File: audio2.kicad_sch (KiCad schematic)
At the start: 10 parts, among them J10 AudioJack3_SwitchTR, J7 AudioJack3_SwitchTR, U3 LM4950TS

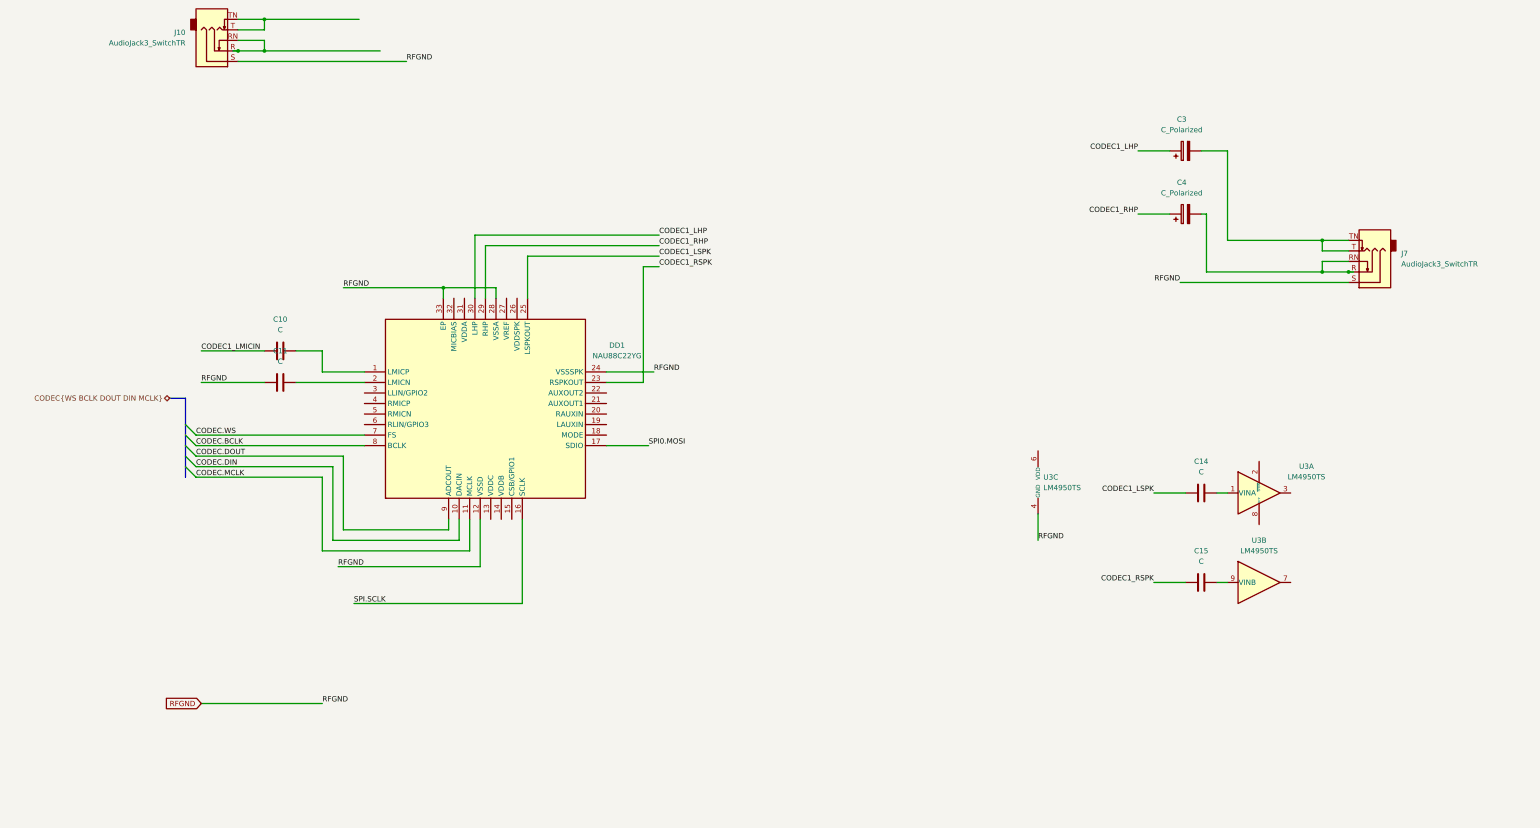
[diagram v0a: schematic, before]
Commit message: Перевёл на иерархические схемы
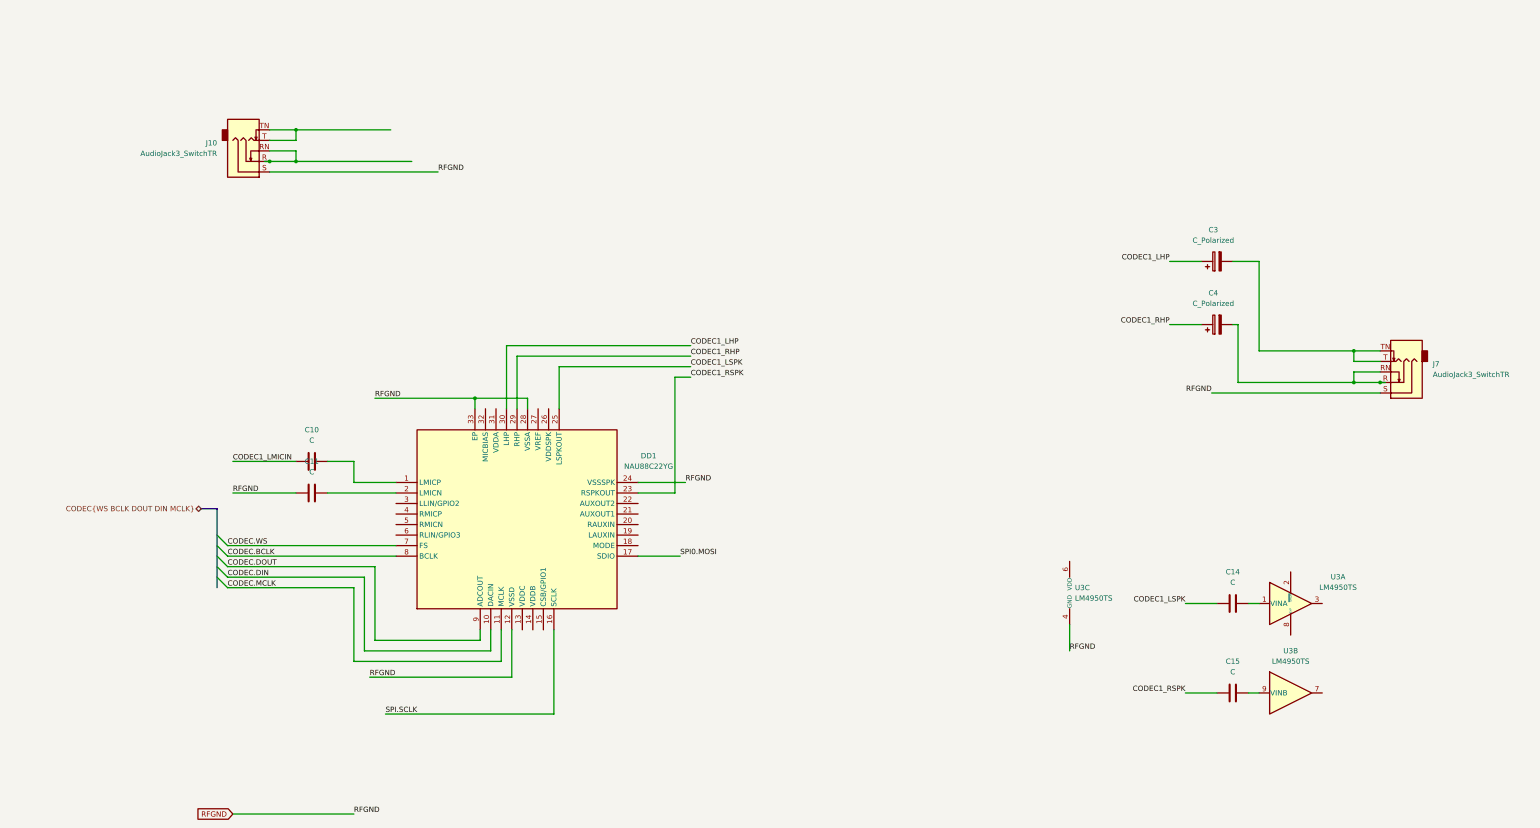
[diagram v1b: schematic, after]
